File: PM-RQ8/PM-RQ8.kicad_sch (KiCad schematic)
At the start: 29 parts, among them J1 2EDGK-5.08-02P, J17 2EDGR-5.08-18P, J2 2EDGK-5.08-02P, J20 Conn_01x03, J21 Conn_01x03, J22 Conn_01x03, J25 Conn_02x08_socket, J3 2EDGK-5.08-02P, J4 2EDGK-5.08-02P, J5 2EDGK-5.08-02P, J6 2EDGK-5.08-02P, J7 2EDGK-5.08-02P, J8 2EDGK-5.08-02P, J9 PinHeader P2.54 01x08 THT Ang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, K1 G5NB-1A-E-DC5, K2 G5NB-1A-E-DC5, K3 G5NB-1A-E-DC5, K4 G5NB-1A-E-DC5, K5 G5NB-1A-E-DC5, K6 G5NB-1A-E-DC5, K7 G5NB-1A-E-DC5, K8 G5NB-1A-E-DC5, U1 ULN2803A, U2 PCA9555PW, U3 64900001039

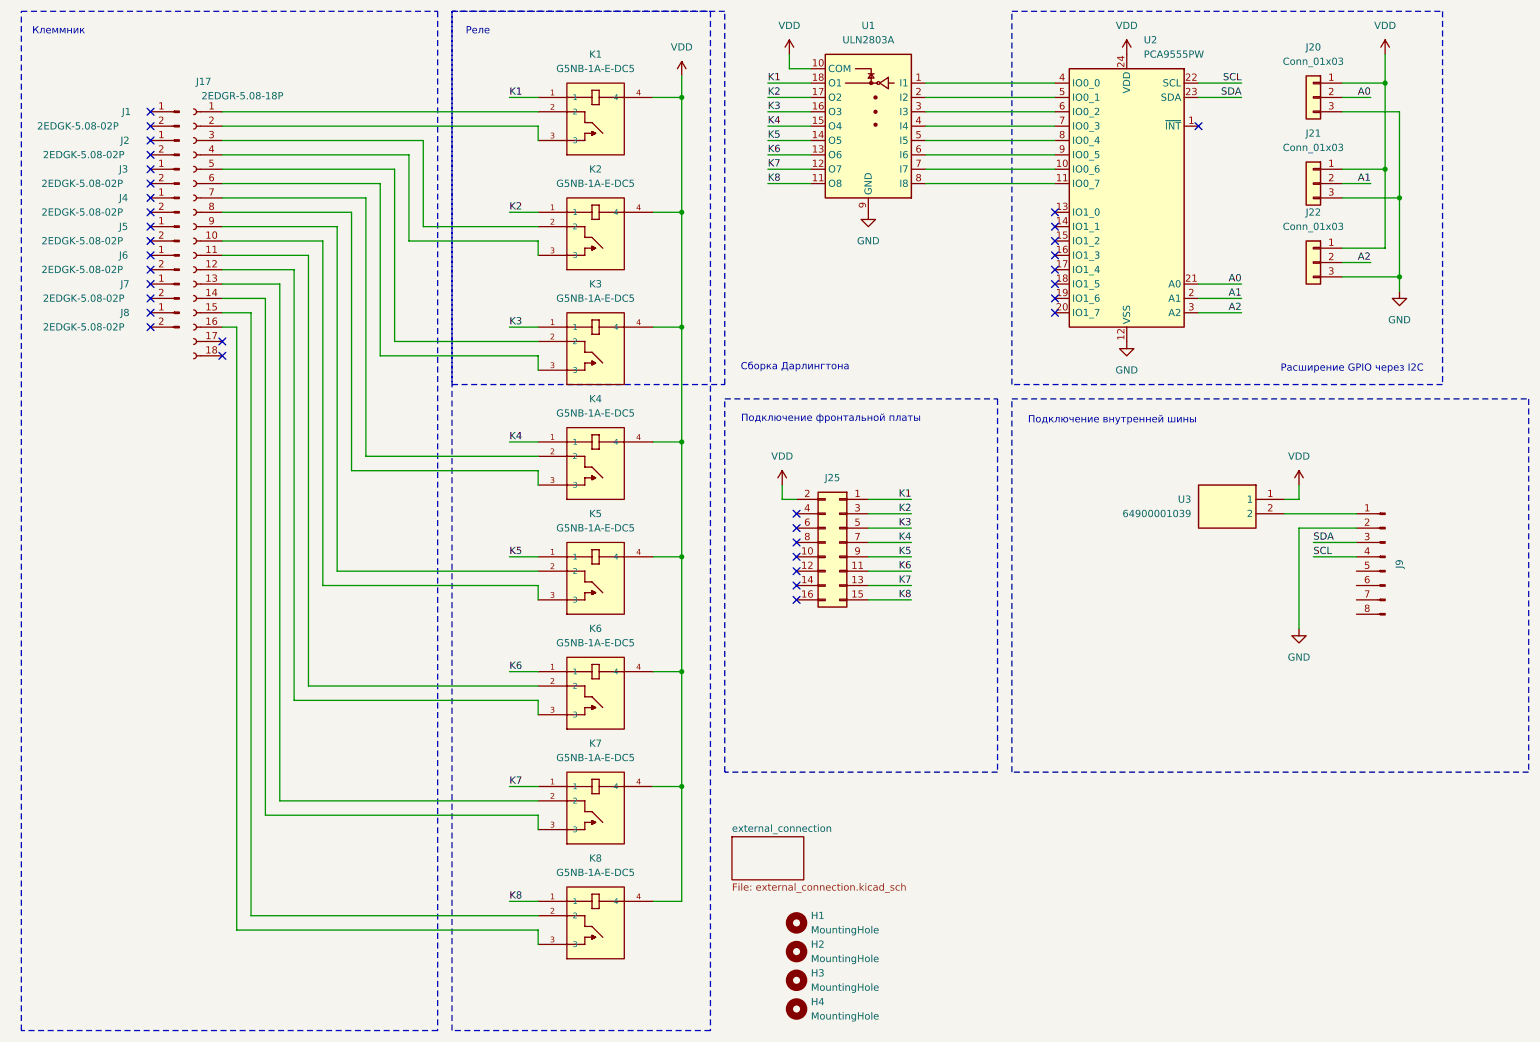
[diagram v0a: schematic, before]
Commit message: PM-RQ8
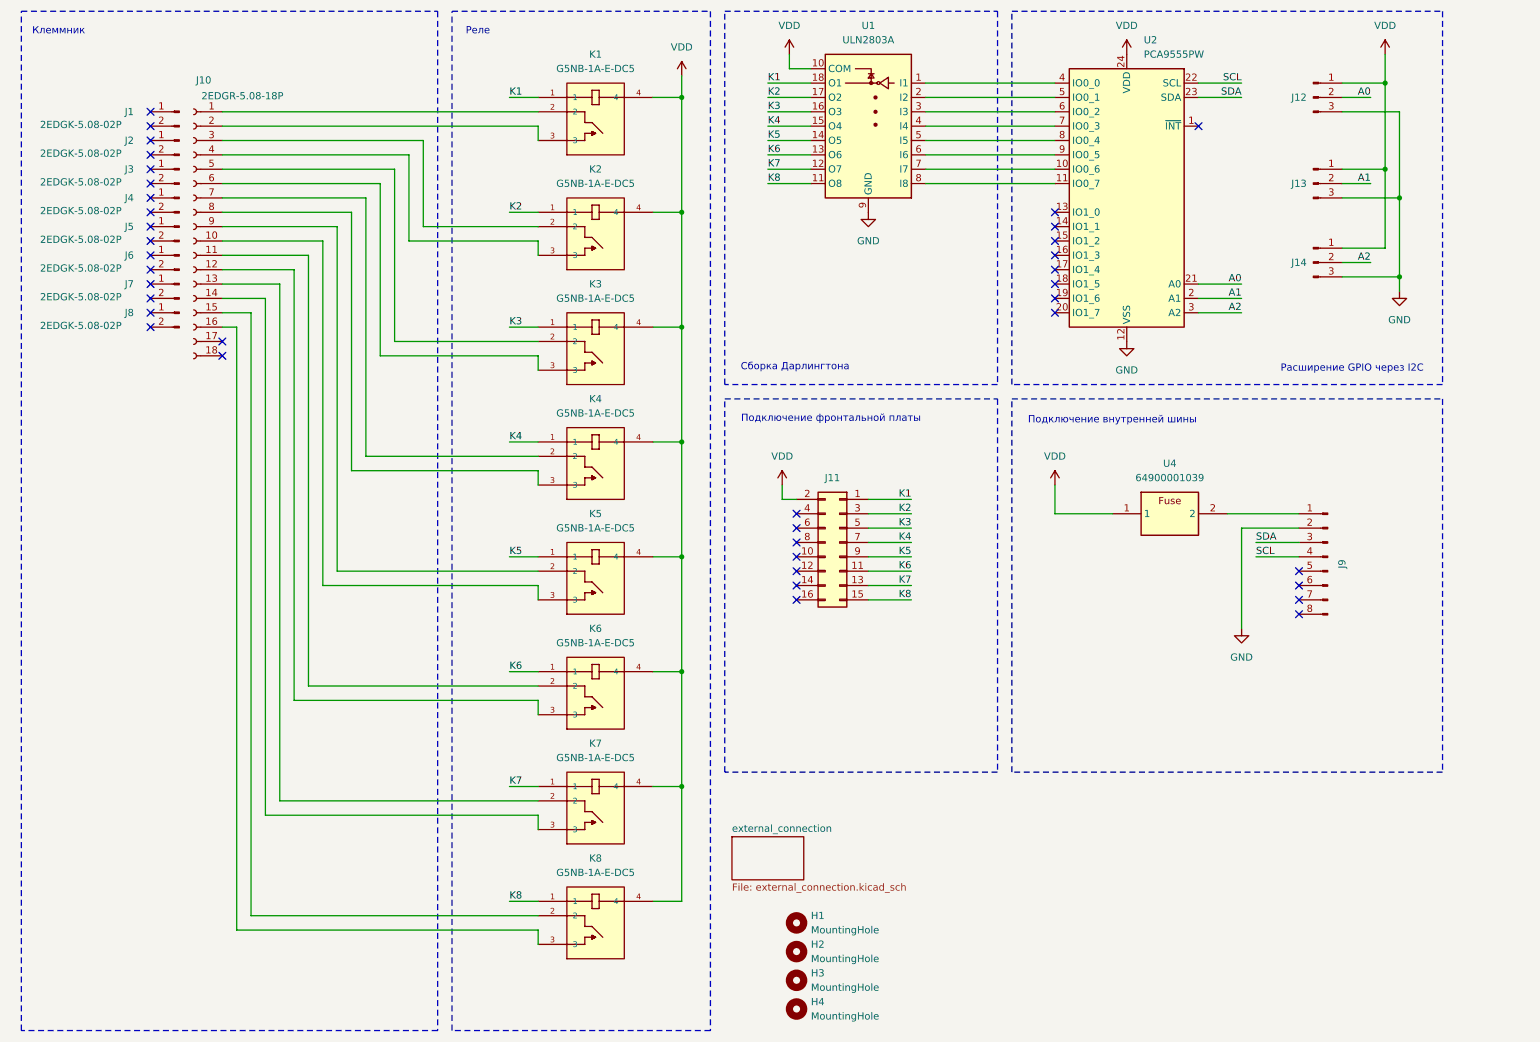
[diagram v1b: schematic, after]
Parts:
- removed J1, J2, J3, J4, J5, J6, J7, J8: 2EDGK-5.08-02P, symbol NextPCB:Degson_2EDGK-5.08-02P
- removed J17: 2EDGR-5.08-18P, NextPCB:Degson_2EDGR-5.08-18P, symbol NextPCB:Degson_2EDGR-5.08-18P
- removed J20, J21, J22: Conn_01x03, Connector_PinHeader_2.54mm:PinHeader_1x03_P2.54mm_Vertical_SMD_Pin1Left, symbol Connector_Generic:Conn_01x03
- removed J25: Conn_02x08_socket, Connector_PinSocket_2.54mm:PinSocket_2x08_P2.54mm_Vertical_SMD, symbol NextPCB:Conn_02x08_socket
- removed U1: ULN2803A, NextPCB:ULN2803A, symbol NextPCB:ULN2803A
- removed U2: PCA9555PW, Package_SO:TSSOP-24_4.4x7.8mm_P0.65mm, symbol NextPCB:PCA9555PW
- removed U3: 64900001039, NextPCB:Fuseholder, symbol NextPCB:Fuseholder
- added J1, J2, J3, J4, J5, J6, J7, J8: 2EDGK-5.08-02P, symbol kicad_inventree_lib:Degson_2EDGK-5.08-02P
- added J10: 2EDGR-5.08-18P, NextPCB:Degson_2EDGR-5.08-18P, symbol kicad_inventree_lib:Degson_2EDGR-5.08-18P
- added J11: FemaleHeader P2.54 02x08 SMD Straight, Connector_PinSocket_2.54mm:PinSocket_2x08_P2.54mm_Vertical_SMD, symbol kicad_inventree_lib:FemaleHeader P2.54 02x08 SMD Straight
- added J12, J13, J14: PinHeader_P2.54_01x03_SMD_Straight, Connector_PinHeader_2.54mm:PinHeader_1x03_P2.54mm_Vertical_SMD_Pin1Left, symbol kicad_inventree_lib:PinHeader P2.54 01x03 SMD Straight
- added U1: ULN2803A, NextPCB:ULN2803A, symbol kicad_inventree_lib:ULN2803A
- added U2: PCA9555PW, Package_SO:TSSOP-24_4.4x7.8mm_P0.65mm, symbol kicad_inventree_lib:PCA9555PW
- added U4: 64900001039, NextPCB:Fuseholder, symbol kicad_inventree_lib:Fuseholder
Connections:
- net A0: now also J12.2 (Pin_2), U2.21 (A0)
- net A1: now also J13.2 (Pin_2), U2.2 (A1)
- net A2: now also J14.2 (Pin_2), U2.3 (A2)
- net GND: now also J12.3 (Pin_3), J13.3 (Pin_3), J14.3 (Pin_3), U1.9 (GND), U2.12 (VSS)
- net K1: now also J11.1 (Pin_1), U1.18 (O1)
- net K2: now also J11.3 (Pin_3), U1.17 (O2)
- net K3: now also J11.5 (Pin_5), U1.16 (O3)
- net K4: now also J11.7 (Pin_7), U1.15 (O4)
- net K5: now also J11.9 (Pin_9), U1.14 (O5)
- net K6: now also J11.11 (Pin_11), U1.13 (O6)
- net K7: now also J11.13 (Pin_13), U1.12 (O7)
- net K8: now also J11.15 (Pin_15), U1.11 (O8)
- net SCL: now also U2.22 (SCL)
- net SDA: now also U2.23 (SDA)
- net VDD: now also J11.2 (Pin_2), J12.1 (Pin_1), J13.1 (Pin_1), J14.1 (Pin_1), U1.10 (COM), U2.24 (VDD), U4.1
- net at K5.2: now also J10.9 (Pin_9)
- net at K5.3: now also J10.10 (Pin_10)
- net at K3.2: now also J10.5 (Pin_5)
- net at K3.3: now also J10.6 (Pin_6)
- net at K8.2: now also J10.15 (Pin_15)
- net at K8.3: now also J10.16 (Pin_16)
- net at K2.2: now also J10.3 (Pin_3)
- net at K2.3: now also J10.4 (Pin_4)
- net at K4.2: now also J10.7 (Pin_7)
- net at K4.3: now also J10.8 (Pin_8)
- net at K1.2: now also J10.1 (Pin_1)
- net at K1.3: now also J10.2 (Pin_2)
- net at K6.2: now also J10.11 (Pin_11)
- net at K6.3: now also J10.12 (Pin_12)
- net at K7.2: now also J10.13 (Pin_13)
- net at K7.3: now also J10.14 (Pin_14)
- net at J9.1 (Pin_1): now also U4.2
- new net: U1.1 (I1), U2.4 (IO0_0)
- new net: U1.2 (I2), U2.5 (IO0_1)
- new net: U1.3 (I3), U2.6 (IO0_2)
- new net: U1.4 (I4), U2.7 (IO0_3)
- new net: U1.5 (I5), U2.8 (IO0_4)
- new net: U1.6 (I6), U2.9 (IO0_5)
- new net: U1.7 (I7), U2.10 (IO0_6)
- new net: U1.8 (I8), U2.11 (IO0_7)
- no-connect marks 34 -> 38
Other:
- moved on the sheet: J9
